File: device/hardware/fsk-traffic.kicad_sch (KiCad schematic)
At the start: 38 parts, among them J1 JTAG, J2 USB_C, J3 2EDGV-5.08-03P, J4 2EDGV-5.08-03P, J5 2EDGV-5.08-03P, Q1 MMBT5551, Q2 AO3401A, Q3 MMBT5551, Q4 AO3401A, U1 XC6206P332MR, U2 MT3608, U3 STM32F070F6Px, Y1 12MHz

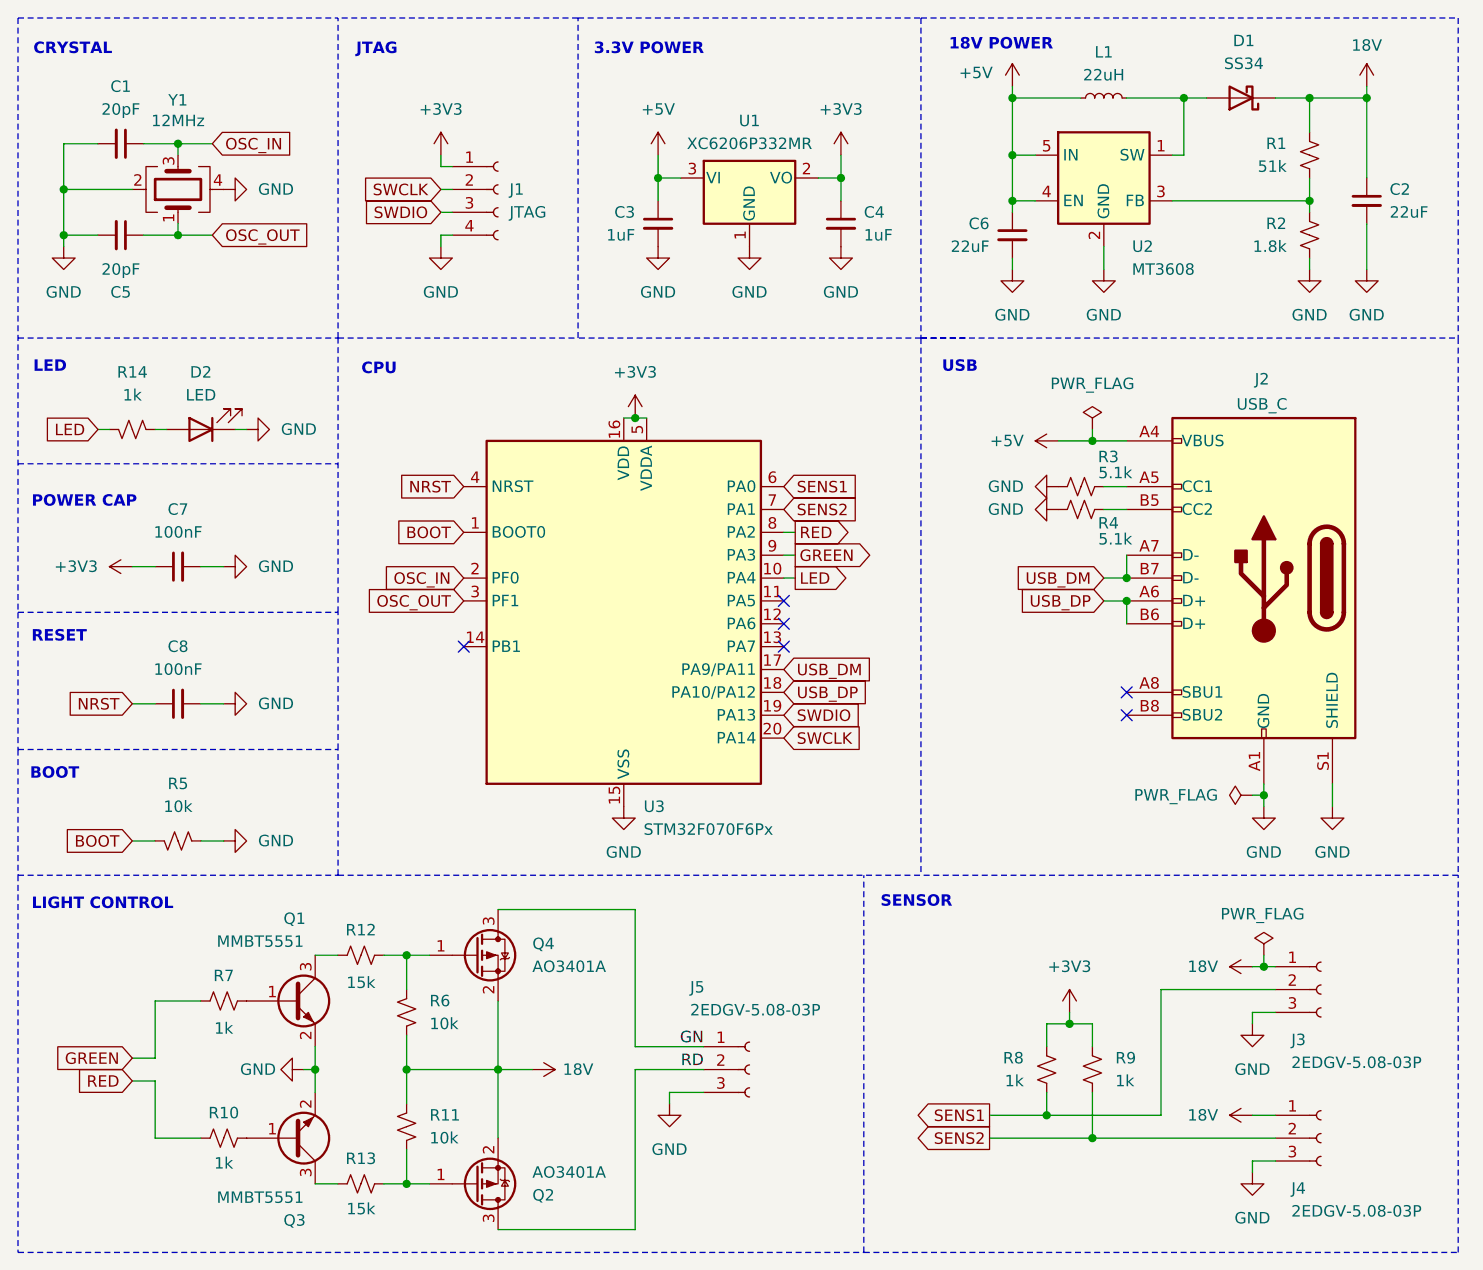
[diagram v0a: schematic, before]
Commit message: fix: isolation & filter
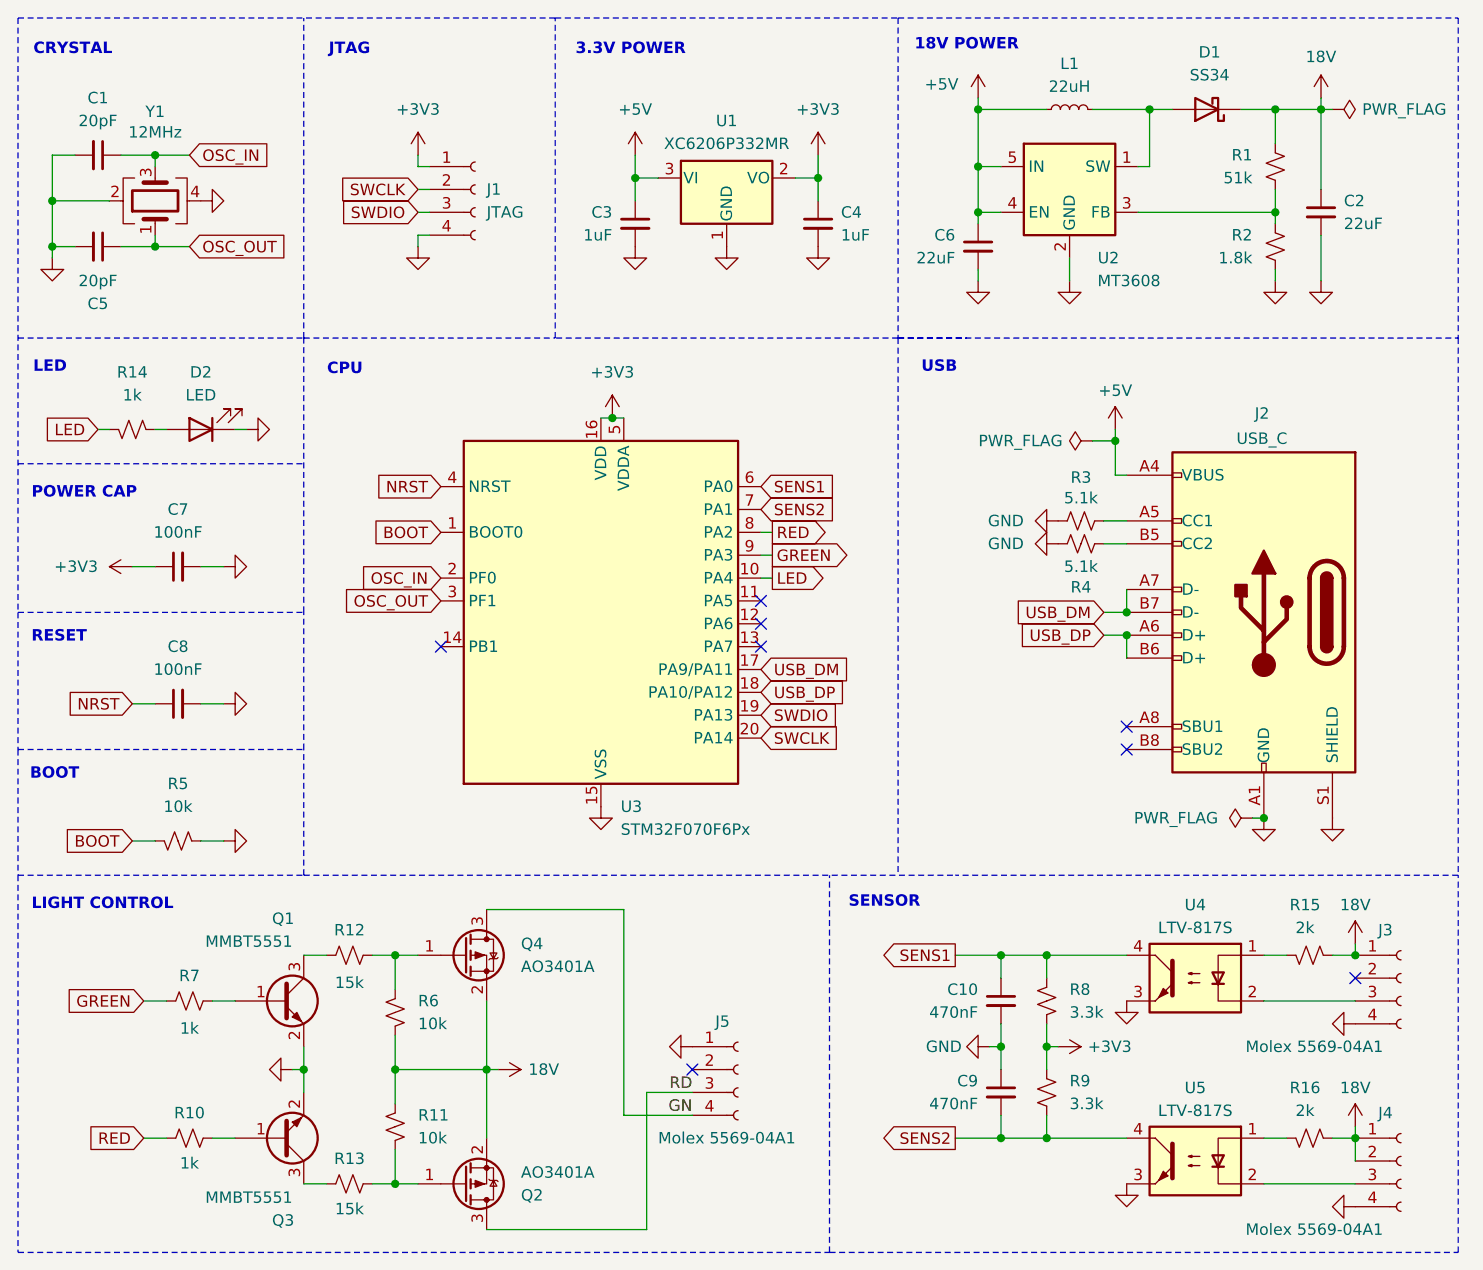
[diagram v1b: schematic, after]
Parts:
- removed J3, J4, J5: 2EDGV-5.08-03P, TerminalBlock_Phoenix:TerminalBlock_Phoenix_MKDS-1,5-3-5.08_1x03_P5.08mm_Horizontal, symbol Connector:Conn_01x03_Socket
- added C10, C9: 470nF, Capacitor_SMD:C_0603_1608Metric, symbol Device:C_Small
- added J3, J4, J5: Molex 5569-04A1, Connector_Molex:Molex_Mini-Fit_Jr_5569-04A1_2x02_P4.20mm_Horizontal, symbol Connector:Conn_01x04_Socket
- added R15, R16: 2k, Resistor_SMD:R_0603_1608Metric, symbol Device:R_Small_US
- added U4, U5: LTV-817S, Package_DIP:SMDIP-4_W9.53mm, symbol Isolator:LTV-817S
- R8, R9: value 1k -> 3.3k; LCSC C21190 -> C22978
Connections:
- net +3V3: now also R8.2; no longer R8.1
- net 18V: now also J3.1 (Pin_1), J4.1 (Pin_1), J4.2 (Pin_2), R15.1, R16.1
- net GN: now also J5.4 (Pin_4)
- net GND: now also C10.2, C9.1, J3.4 (Pin_4), J4.4 (Pin_4), J5.1 (Pin_1), U4.3, U5.3
- net RD: now also J5.3 (Pin_3)
- net SENS1: now also R8.1, C10.1, U4.4; no longer R8.2
- net SENS2: now also C9.2, U5.4
- new net: J4.3 (Pin_3), U5.2
- new net: R15.2, U4.1
- new net: R16.2, U5.1
- new net: J3.3 (Pin_3), U4.2
- no-connect marks 6 -> 8
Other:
- moved on the sheet: C1, C2, C3, C4, C5, C6, D1, J1, J2, L1, Q1, Q2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
